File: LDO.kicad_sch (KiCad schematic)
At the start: 3 parts, among them U1 AMS1117-3.3

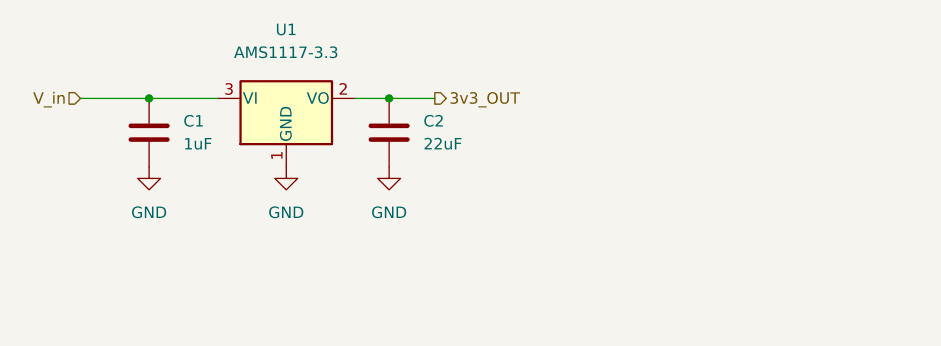
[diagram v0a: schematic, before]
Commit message: Updated subsheets
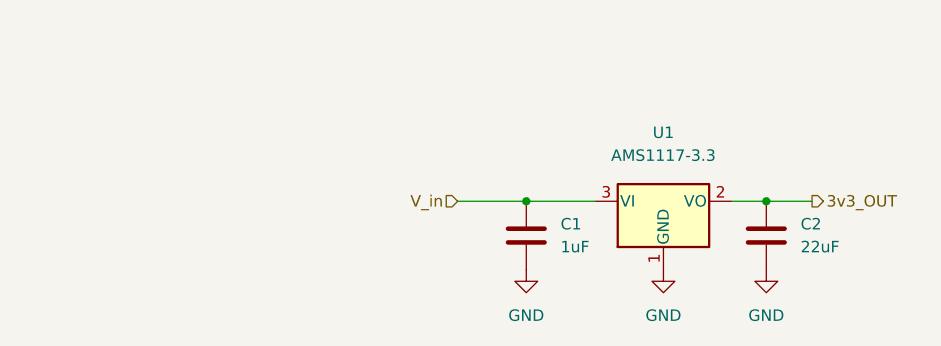
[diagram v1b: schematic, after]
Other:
- moved on the sheet: C1, C2, U1
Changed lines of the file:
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@@
 (kicad_sch (version 20211123) (generator eeschema)
   (paper "A4")
-  (junction (at 96.52 83.82) (diameter 0) (color 0 0 0 0)
+  (junction (at 138.43 95.25) (diameter 0) (color 0 0 0 0)
   )
-  (junction (at 123.19 83.82) (diameter 0) (color 0 0 0 0)
+  (junction (at 165.1 95.25) (diameter 0) (color 0 0 0 0)
   )
-  (wire (pts (xy 123.19 83.82) (xy 119.38 83.82))
+  (wire (pts (xy 165.1 95.25) (xy 161.29 95.25))
     (stroke (width 0) (type default) (color 0 0 0 0))
   )
-  (wire (pts (xy 88.9 83.82) (xy 96.52 83.82))
+  (wire (pts (xy 130.81 95.25) (xy 138.43 95.25))
     (stroke (width 0) (type default) (color 0 0 0 0))
   )
-  (wire (pts (xy 96.52 83.82) (xy 104.14 83.82))
+  (wire (pts (xy 138.43 95.25) (xy 146.05 95.25))
     (stroke (width 0) (type default) (color 0 0 0 0))
   )
-  (wire (pts (xy 128.27 83.82) (xy 123.19 83.82))
+  (wire (pts (xy 170.18 95.25) (xy 165.1 95.25))
     (stroke (width 0) (type default) (color 0 0 0 0))
   )
-  (hierarchical_label "V_in" (shape input) (at 88.9 83.82 180)
+  (hierarchical_label "V_in" (shape input) (at 130.81 95.25 180)
     (effects (font (size 1.27 1.27)) (justify right))
   )
-  (hierarchical_label "3v3_OUT" (shape output) (at 128.27 83.82 0)
+  (hierarchical_label "3v3_OUT" (shape output) (at 170.18 95.25 0)
     (effects (font (size 1.27 1.27)) (justify left))
   )
-  (symbol (lib_id "power:GND") (at 96.52 91.44 0) (unit 1)
+  (symbol (lib_id "power:GND") (at 138.43 102.87 0) (unit 1)
     (in_bom yes) (on_board yes) (fields_autoplaced)
-    (property "Reference" "#PWR01" (id 0) (at 96.52 97.79 0)
+    (property "Reference" "#PWR01" (id 0) (at 138.43 109.22 0)
       (effects (font (size 1.27 1.27)) hide)
     )
-    (property "Value" "GND" (id 1) (at 96.52 96.52 0))
-    (property "Footprint" "" (id 2) (at 96.52 91.44 0)
+    (property "Value" "GND" (id 1) (at 138.43 107.95 0))
+    (property "Footprint" "" (id 2) (at 138.43 102.87 0)
       (effects (font (size 1.27 1.27)) hide)
     )
-    (property "Datasheet" "" (id 3) (at 96.52 91.44 0)
+    (property "Datasheet" "" (id 3) (at 138.43 102.87 0)
       (effects (font (size 1.27 1.27)) hide)
     )
     (pin "1")
   )
-  (symbol (lib_id "Device:C") (at 123.19 87.63 0) (unit 1)
+  (symbol (lib_id "Device:C") (at 165.1 99.06 0) (unit 1)
     (in_bom yes) (on_board yes) (fields_autoplaced)
-    (property "Reference" "C2" (id 0) (at 127 86.3599 0)
+    (property "Reference" "C2" (id 0) (at 168.91 97.7899 0)
       (effects (font (size 1.27 1.27)) (justify left))
     )
-    (property "Value" "22uF" (id 1) (at 127 88.8999 0)
+    (property "Value" "22uF" (id 1) (at 168.91 100.3299 0)
       (effects (font (size 1.27 1.27)) (justify left))
     )
-    (property "Footprint" "Capacitor_SMD:C_0603_1608Metric_Pad1.08x0.95mm_HandSolder" (id 2) (at 124.1552 91.44 0)
+    (property "Footprint" "Capacitor_SMD:C_0603_1608Metric_Pad1.08x0.95mm_HandSolder" (id 2) (at 166.0652 102.87 0)
       (effects (font (size 1.27 1.27)) hide)
     )
-    (property "Datasheet" "~" (id 3) (at 123.19 87.63 0)
+    (property "Datasheet" "~" (id 3) (at 165.1 99.06 0)
       (effects (font (size 1.27 1.27)) hide)
     )
@@
     (pin "2")
   )
-  (symbol (lib_id "power:GND") (at 111.76 91.44 0) (unit 1)
+  (symbol (lib_id "power:GND") (at 153.67 102.87 0) (unit 1)
     (in_bom yes) (on_board yes) (fields_autoplaced)
-    (property "Reference" "#PWR02" (id 0) (at 111.76 97.79 0)
+    (property "Reference" "#PWR02" (id 0) (at 153.67 109.22 0)
       (effects (font (size 1.27 1.27)) hide)
     )
-    (property "Value" "GND" (id 1) (at 111.76 96.52 0))
-    (property "Footprint" "" (id 2) (at 111.76 91.44 0)
+    (property "Value" "GND" (id 1) (at 153.67 107.95 0))
+    (property "Footprint" "" (id 2) (at 153.67 102.87 0)
       (effects (font (size 1.27 1.27)) hide)
     )
-    (property "Datasheet" "" (id 3) (at 111.76 91.44 0)
+    (property "Datasheet" "" (id 3) (at 153.67 102.87 0)
       (effects (font (size 1.27 1.27)) hide)
     )
     (pin "1")
   )
-  (symbol (lib_id "power:GND") (at 123.19 91.44 0) (unit 1)
+  (symbol (lib_id "power:GND") (at 165.1 102.87 0) (unit 1)
     (in_bom yes) (on_board yes) (fields_autoplaced)
-    (property "Reference" "#PWR03" (id 0) (at 123.19 97.79 0)
+    (property "Reference" "#PWR03" (id 0) (at 165.1 109.22 0)
       (effects (font (size 1.27 1.27)) hide)
     )
-    (property "Value" "GND" (id 1) (at 123.19 96.52 0))
-    (property "Footprint" "" (id 2) (at 123.19 91.44 0)
+    (property "Value" "GND" (id 1) (at 165.1 107.95 0))
+    (property "Footprint" "" (id 2) (at 165.1 102.87 0)
       (effects (font (size 1.27 1.27)) hide)
     )
-    (property "Datasheet" "" (id 3) (at 123.19 91.44 0)
+    (property "Datasheet" "" (id 3) (at 165.1 102.87 0)
       (effects (font (size 1.27 1.27)) hide)
     )
     (pin "1")
   )
-  (symbol (lib_id "Device:C") (at 96.52 87.63 0) (unit 1)
+  (symbol (lib_id "Device:C") (at 138.43 99.06 0) (unit 1)
     (in_bom yes) (on_board yes) (fields_autoplaced)
-    (property "Reference" "C1" (id 0) (at 100.33 86.3599 0)
+    (property "Reference" "C1" (id 0) (at 142.24 97.7899 0)
       (effects (font (size 1.27 1.27)) (justify left))
     )
-    (property "Value" "1uF" (id 1) (at 100.33 88.8999 0)
+    (property "Value" "1uF" (id 1) (at 142.24 100.3299 0)
       (effects (font (size 1.27 1.27)) (justify left))
     )
-    (property "Footprint" "Capacitor_SMD:C_0603_1608Metric_Pad1.08x0.95mm_HandSolder" (id 2) (at 97.4852 91.44 0)
+    (property "Footprint" "Capacitor_SMD:C_0603_1608Metric_Pad1.08x0.95mm_HandSolder" (id 2) (at 139.3952 102.87 0)
       (effects (font (size 1.27 1.27)) hide)
     )
-    (property "Datasheet" "~" (id 3) (at 96.52 87.63 0)
+    (property "Datasheet" "~" (id 3) (at 138.43 99.06 0)
       (effects (font (size 1.27 1.27)) hide)
     )
@@
     (pin "2")
   )
-  (symbol (lib_id "Regulator_Linear:AMS1117-3.3") (at 111.76 83.82 0) (unit 1)
+  (symbol (lib_id "Regulator_Linear:AMS1117-3.3") (at 153.67 95.25 0) (unit 1)
     (in_bom yes) (on_board yes) (fields_autoplaced)
-    (property "Reference" "U1" (id 0) (at 111.76 76.2 0))
-    (property "Value" "AMS1117-3.3" (id 1) (at 111.76 78.74 0))
-    (property "Footprint" "Package_TO_SOT_SMD:SOT-223-3_TabPin2" (id 2) (at 111.76 78.74 0)
+    (property "Reference" "U1" (id 0) (at 153.67 87.63 0))
+    (property "Value" "AMS1117-3.3" (id 1) (at 153.67 90.17 0))
+    (property "Footprint" "Package_TO_SOT_SMD:SOT-223-3_TabPin2" (id 2) (at 153.67 90.17 0)
       (effects (font (size 1.27 1.27)) hide)
     )
-    (property "Datasheet" "http://www.advanced-monolithic.com/pdf/ds1117.pdf" (id 3) (at 114.3 90.17 0)
+    (property "Datasheet" "http://www.advanced-monolithic.com/pdf/ds1117.pdf" (id 3) (at 156.21 101.6 0)
       (effects (font (size 1.27 1.27)) hide)
     )

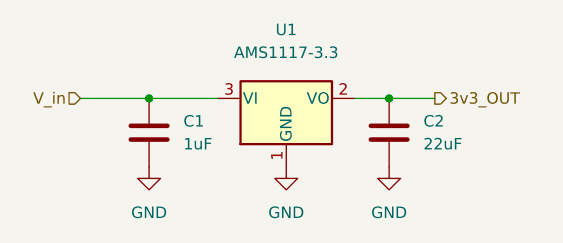
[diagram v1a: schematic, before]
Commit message: Updated (?) subsheets
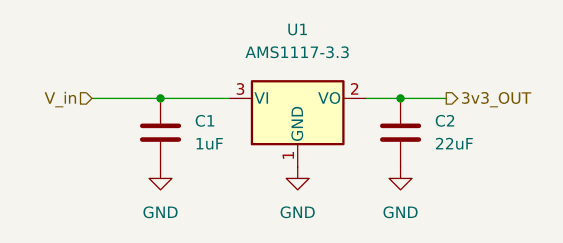
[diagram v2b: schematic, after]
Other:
- moved on the sheet: C1, C2, U1
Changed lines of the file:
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@@
 (kicad_sch (version 20211123) (generator eeschema)
   (paper "A4")
-  (junction (at 138.43 95.25) (diameter 0) (color 0 0 0 0)
+  (junction (at 139.7 95.25) (diameter 0) (color 0 0 0 0)
   )
-  (junction (at 165.1 95.25) (diameter 0) (color 0 0 0 0)
+  (junction (at 166.37 95.25) (diameter 0) (color 0 0 0 0)
   )
-  (wire (pts (xy 165.1 95.25) (xy 161.29 95.25))
+  (wire (pts (xy 166.37 95.25) (xy 162.56 95.25))
     (stroke (width 0) (type default) (color 0 0 0 0))
   )
-  (wire (pts (xy 130.81 95.25) (xy 138.43 95.25))
+  (wire (pts (xy 132.08 95.25) (xy 139.7 95.25))
     (stroke (width 0) (type default) (color 0 0 0 0))
   )
-  (wire (pts (xy 138.43 95.25) (xy 146.05 95.25))
+  (wire (pts (xy 139.7 95.25) (xy 147.32 95.25))
     (stroke (width 0) (type default) (color 0 0 0 0))
   )
-  (wire (pts (xy 170.18 95.25) (xy 165.1 95.25))
+  (wire (pts (xy 171.45 95.25) (xy 166.37 95.25))
     (stroke (width 0) (type default) (color 0 0 0 0))
   )
-  (hierarchical_label "V_in" (shape input) (at 130.81 95.25 180)
+  (hierarchical_label "V_in" (shape input) (at 132.08 95.25 180)
     (effects (font (size 1.27 1.27)) (justify right))
   )
-  (hierarchical_label "3v3_OUT" (shape output) (at 170.18 95.25 0)
+  (hierarchical_label "3v3_OUT" (shape output) (at 171.45 95.25 0)
     (effects (font (size 1.27 1.27)) (justify left))
   )
-  (symbol (lib_id "power:GND") (at 138.43 102.87 0) (unit 1)
+  (symbol (lib_id "power:GND") (at 139.7 102.87 0) (unit 1)
     (in_bom yes) (on_board yes) (fields_autoplaced)
-    (property "Reference" "#PWR01" (id 0) (at 138.43 109.22 0)
+    (property "Reference" "#PWR01" (id 0) (at 139.7 109.22 0)
       (effects (font (size 1.27 1.27)) hide)
     )
-    (property "Value" "GND" (id 1) (at 138.43 107.95 0))
-    (property "Footprint" "" (id 2) (at 138.43 102.87 0)
+    (property "Value" "GND" (id 1) (at 139.7 107.95 0))
+    (property "Footprint" "" (id 2) (at 139.7 102.87 0)
       (effects (font (size 1.27 1.27)) hide)
     )
-    (property "Datasheet" "" (id 3) (at 138.43 102.87 0)
+    (property "Datasheet" "" (id 3) (at 139.7 102.87 0)
       (effects (font (size 1.27 1.27)) hide)
     )
     (pin "1")
   )
-  (symbol (lib_id "Device:C") (at 165.1 99.06 0) (unit 1)
+  (symbol (lib_id "Device:C") (at 166.37 99.06 0) (unit 1)
     (in_bom yes) (on_board yes) (fields_autoplaced)
-    (property "Reference" "C2" (id 0) (at 168.91 97.7899 0)
+    (property "Reference" "C2" (id 0) (at 170.18 97.7899 0)
       (effects (font (size 1.27 1.27)) (justify left))
     )
-    (property "Value" "22uF" (id 1) (at 168.91 100.3299 0)
+    (property "Value" "22uF" (id 1) (at 170.18 100.3299 0)
       (effects (font (size 1.27 1.27)) (justify left))
     )
-    (property "Footprint" "Capacitor_SMD:C_0603_1608Metric_Pad1.08x0.95mm_HandSolder" (id 2) (at 166.0652 102.87 0)
+    (property "Footprint" "Capacitor_SMD:C_0603_1608Metric_Pad1.08x0.95mm_HandSolder" (id 2) (at 167.3352 102.87 0)
       (effects (font (size 1.27 1.27)) hide)
     )
-    (property "Datasheet" "~" (id 3) (at 165.1 99.06 0)
+    (property "Datasheet" "~" (id 3) (at 166.37 99.06 0)
       (effects (font (size 1.27 1.27)) hide)
     )
@@
     (pin "2")
   )
-  (symbol (lib_id "power:GND") (at 153.67 102.87 0) (unit 1)
+  (symbol (lib_id "power:GND") (at 154.94 102.87 0) (unit 1)
     (in_bom yes) (on_board yes) (fields_autoplaced)
-    (property "Reference" "#PWR02" (id 0) (at 153.67 109.22 0)
+    (property "Reference" "#PWR02" (id 0) (at 154.94 109.22 0)
       (effects (font (size 1.27 1.27)) hide)
     )
-    (property "Value" "GND" (id 1) (at 153.67 107.95 0))
-    (property "Footprint" "" (id 2) (at 153.67 102.87 0)
+    (property "Value" "GND" (id 1) (at 154.94 107.95 0))
+    (property "Footprint" "" (id 2) (at 154.94 102.87 0)
       (effects (font (size 1.27 1.27)) hide)
     )
-    (property "Datasheet" "" (id 3) (at 153.67 102.87 0)
+    (property "Datasheet" "" (id 3) (at 154.94 102.87 0)
       (effects (font (size 1.27 1.27)) hide)
     )
     (pin "1")
   )
-  (symbol (lib_id "power:GND") (at 165.1 102.87 0) (unit 1)
+  (symbol (lib_id "power:GND") (at 166.37 102.87 0) (unit 1)
     (in_bom yes) (on_board yes) (fields_autoplaced)
-    (property "Reference" "#PWR03" (id 0) (at 165.1 109.22 0)
+    (property "Reference" "#PWR03" (id 0) (at 166.37 109.22 0)
       (effects (font (size 1.27 1.27)) hide)
     )
-    (property "Value" "GND" (id 1) (at 165.1 107.95 0))
-    (property "Footprint" "" (id 2) (at 165.1 102.87 0)
+    (property "Value" "GND" (id 1) (at 166.37 107.95 0))
+    (property "Footprint" "" (id 2) (at 166.37 102.87 0)
       (effects (font (size 1.27 1.27)) hide)
     )
-    (property "Datasheet" "" (id 3) (at 165.1 102.87 0)
+    (property "Datasheet" "" (id 3) (at 166.37 102.87 0)
       (effects (font (size 1.27 1.27)) hide)
     )
     (pin "1")
   )
-  (symbol (lib_id "Device:C") (at 138.43 99.06 0) (unit 1)
+  (symbol (lib_id "Device:C") (at 139.7 99.06 0) (unit 1)
     (in_bom yes) (on_board yes) (fields_autoplaced)
-    (property "Reference" "C1" (id 0) (at 142.24 97.7899 0)
+    (property "Reference" "C1" (id 0) (at 143.51 97.7899 0)
       (effects (font (size 1.27 1.27)) (justify left))
     )
-    (property "Value" "1uF" (id 1) (at 142.24 100.3299 0)
+    (property "Value" "1uF" (id 1) (at 143.51 100.3299 0)
       (effects (font (size 1.27 1.27)) (justify left))
     )
-    (property "Footprint" "Capacitor_SMD:C_0603_1608Metric_Pad1.08x0.95mm_HandSolder" (id 2) (at 139.3952 102.87 0)
+    (property "Footprint" "Capacitor_SMD:C_0603_1608Metric_Pad1.08x0.95mm_HandSolder" (id 2) (at 140.6652 102.87 0)
       (effects (font (size 1.27 1.27)) hide)
     )
-    (property "Datasheet" "~" (id 3) (at 138.43 99.06 0)
+    (property "Datasheet" "~" (id 3) (at 139.7 99.06 0)
       (effects (font (size 1.27 1.27)) hide)
     )
@@
     (pin "2")
   )
-  (symbol (lib_id "Regulator_Linear:AMS1117-3.3") (at 153.67 95.25 0) (unit 1)
+  (symbol (lib_id "Regulator_Linear:AMS1117-3.3") (at 154.94 95.25 0) (unit 1)
     (in_bom yes) (on_board yes) (fields_autoplaced)
-    (property "Reference" "U1" (id 0) (at 153.67 87.63 0))
-    (property "Value" "AMS1117-3.3" (id 1) (at 153.67 90.17 0))
-    (property "Footprint" "Package_TO_SOT_SMD:SOT-223-3_TabPin2" (id 2) (at 153.67 90.17 0)
+    (property "Reference" "U1" (id 0) (at 154.94 87.63 0))
+    (property "Value" "AMS1117-3.3" (id 1) (at 154.94 90.17 0))
+    (property "Footprint" "Package_TO_SOT_SMD:SOT-223-3_TabPin2" (id 2) (at 154.94 90.17 0)
       (effects (font (size 1.27 1.27)) hide)
     )
-    (property "Datasheet" "http://www.advanced-monolithic.com/pdf/ds1117.pdf" (id 3) (at 156.21 101.6 0)
+    (property "Datasheet" "http://www.advanced-monolithic.com/pdf/ds1117.pdf" (id 3) (at 157.48 101.6 0)
       (effects (font (size 1.27 1.27)) hide)
     )
